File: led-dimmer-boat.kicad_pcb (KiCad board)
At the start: 2 copper layers, 62 x 30 mm, 18 parts, among them J1 PWR, J2 Prog, J3 LEDSTRIP, Q1 IRLB8721PBF, Q2 IRLB8721PBF, Q4 2N3904, SW1 M2023SS1W03, U1 ATtiny13A-PU-ND, U2 LM7805S/NOPB

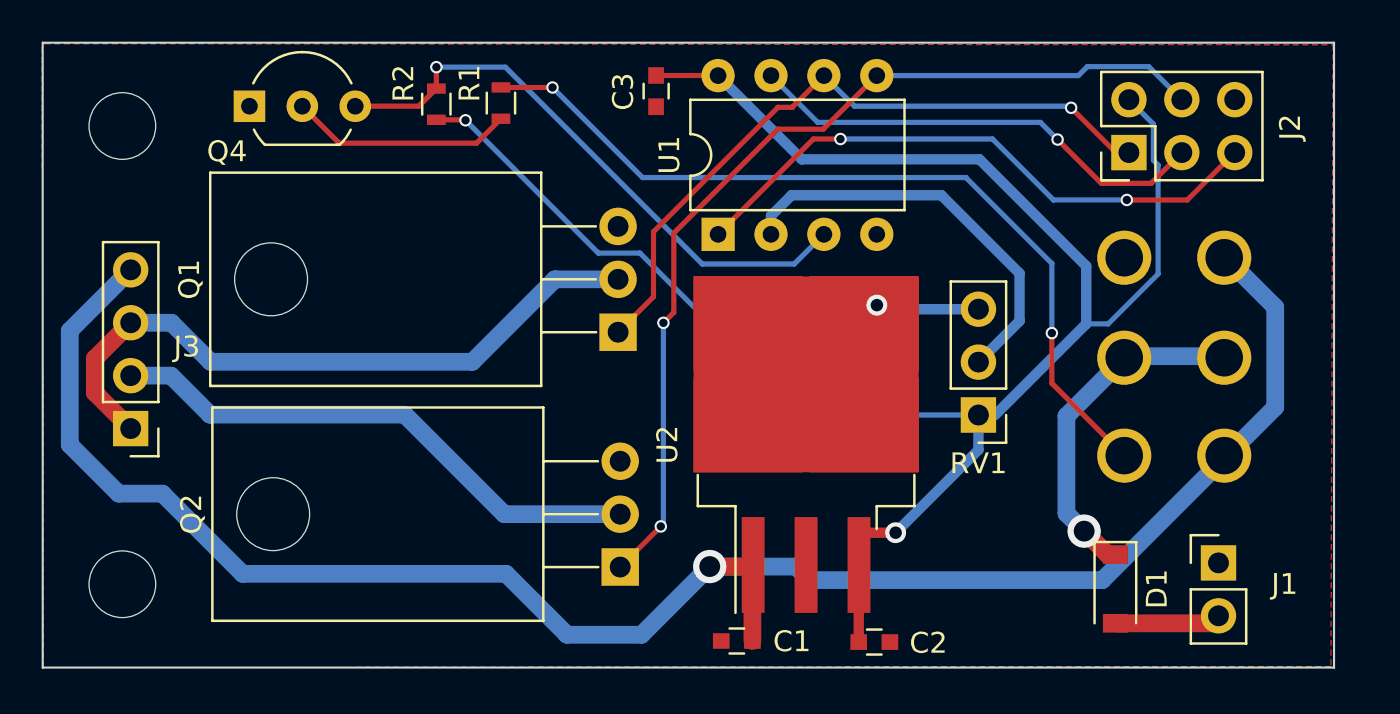
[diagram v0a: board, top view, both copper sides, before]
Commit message: Updated schematic.pdf and added board.png
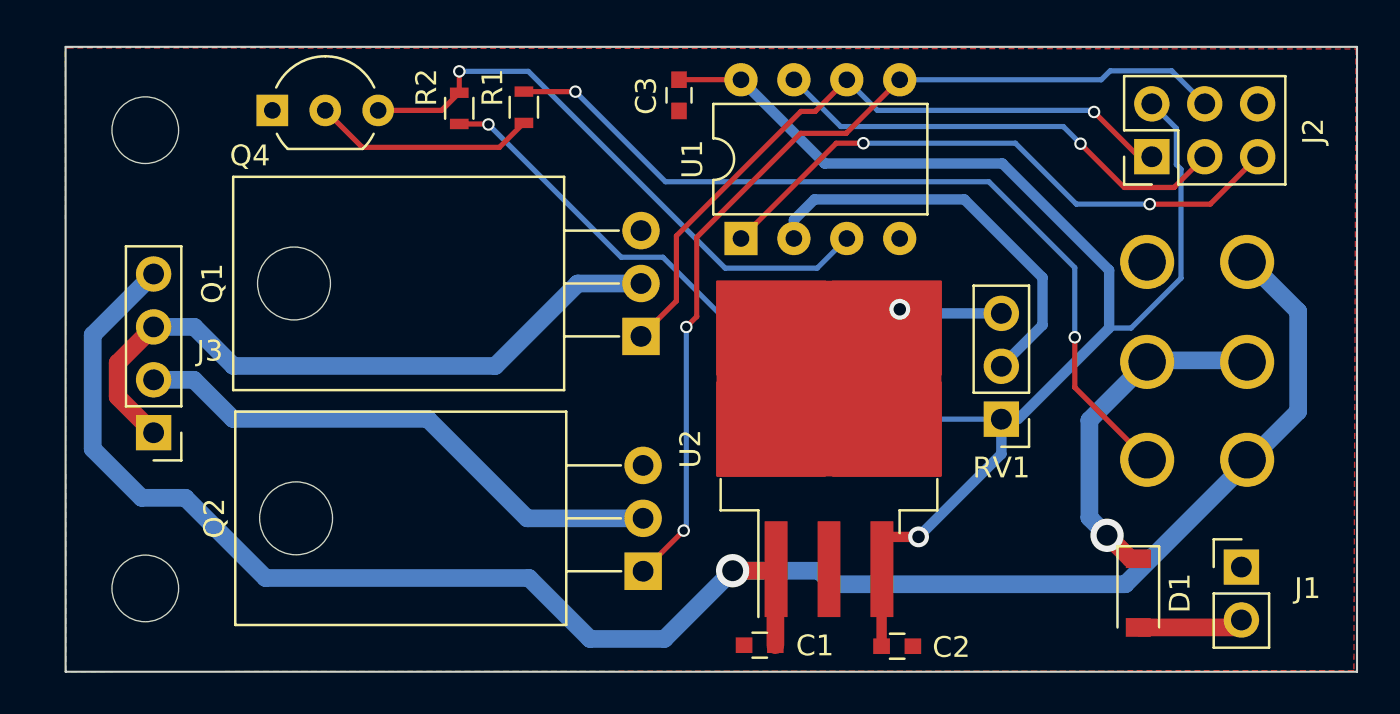
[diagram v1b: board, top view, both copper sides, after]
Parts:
- moved C1 1.12 mm to (134.4, 108.9)
- moved C3 1.12 mm to (130.6, 82.5)
- moved J1 1.12 mm to (157.6, 105.2)
- moved Q4 1.12 mm to (111.0, 83.2)
- moved J3 1.12 mm to (105.3, 98.7)
- moved D1 1.12 mm to (152.6, 106.4)
- moved H1 1.12 mm to (104.9, 84.2)
- moved H2 1.12 mm to (104.9, 106.2)
- moved Q2 1.12 mm to (128.8, 105.4)
- moved R2 1.12 mm to (120.0, 83.2)
- moved RV1 1.12 mm to (146.0, 98.1)
- moved SW1 1.12 mm to (153.0, 100.0)
- moved U1 1.12 mm to (133.5, 89.4)
- moved U2 1.12 mm to (137.8, 99.5)
- moved C2 1.12 mm to (141.0, 109.0)
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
